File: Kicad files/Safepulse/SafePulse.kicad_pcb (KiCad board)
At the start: 4 copper layers, 40.6 x 20.8 mm, 90 parts, among them J1 Conn_01x03_Male, Q1 FQT7N10L, Q2 BC846A, Q3 MMBT3906, Q4 MMBT3906, U1 TS4061AILT-1.25, U2 74HC14, U3 TLV27L1DBVT, U33 MAX9910EXK+T, U4 CD14538BM

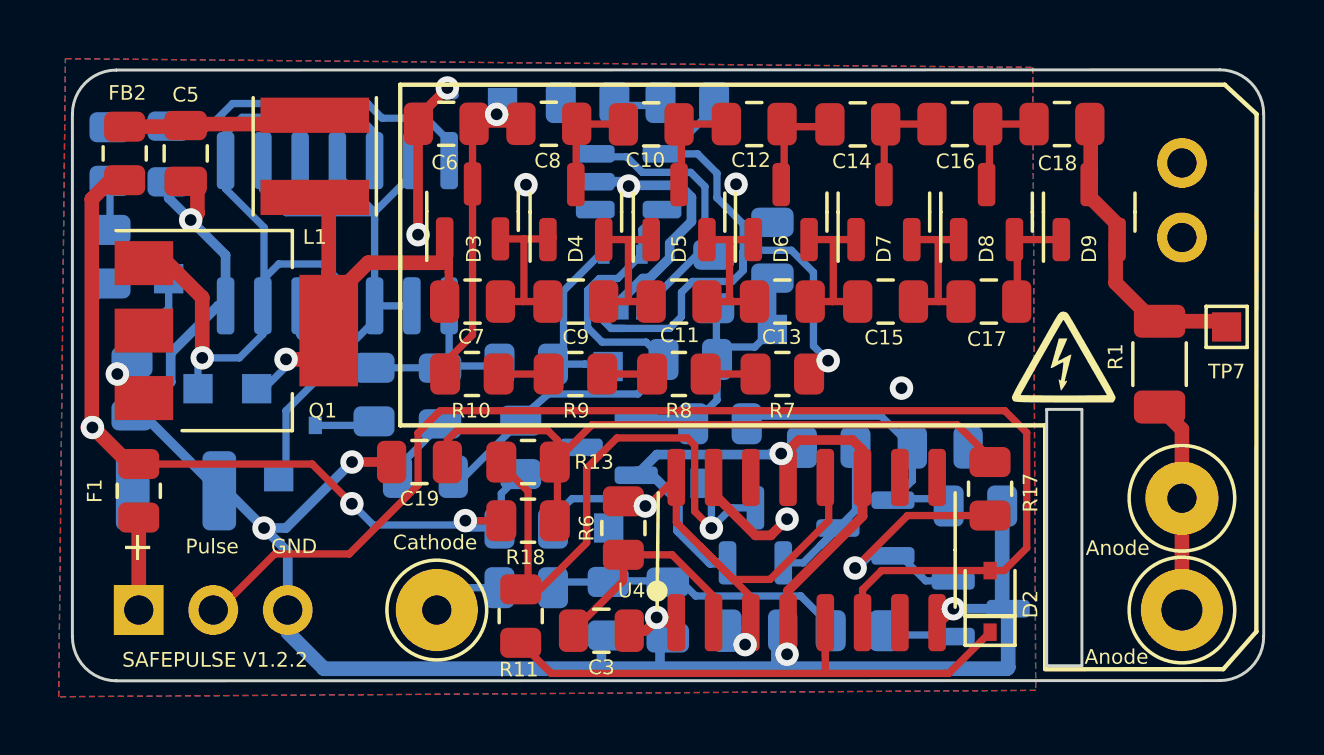
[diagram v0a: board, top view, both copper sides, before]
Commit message: Updated with Gerbers
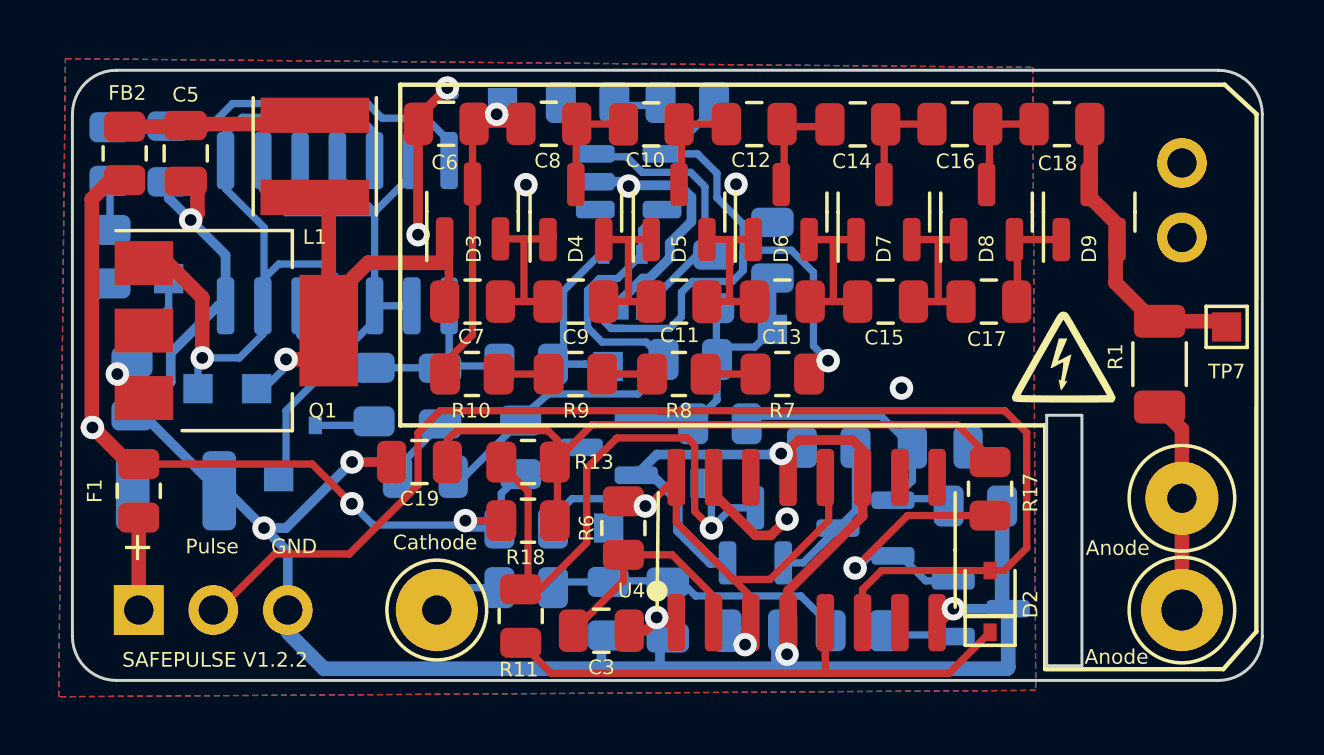
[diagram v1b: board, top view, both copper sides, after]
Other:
- outline, holes or cut-outs redrawn
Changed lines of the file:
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@@
   (gr_line (start 165.52 57.658) (end 137.414 57.658) (layer "F.SilkS") (width 0.15))
   (gr_line (start 165.52 57.658) (end 166.604 58.658) (layer "F.SilkS") (width 0.15))
-  (gr_arc (start 165.347 76.47) (end 166.847 76.47) (angle 90) (layer "Edge.Cuts") (width 0.1))
-  (gr_line (start 165.347 77.97) (end 127.738 77.978) (layer "Edge.Cuts") (width 0.1))
-  (gr_line (start 166.847 58.65) (end 166.847 76.47) (layer "Edge.Cuts") (width 0.1))
-  (gr_arc (start 165.347 58.65) (end 165.347 57.15) (angle 90) (layer "Edge.Cuts") (width 0.1))
-  (gr_rect (start 159.45 68.725) (end 160.65 77.465) (layer "Edge.Cuts") (width 0.1) (fill none))
-  (gr_arc (start 127.738 76.478) (end 127.738 77.978) (angle 90) (layer "Edge.Cuts") (width 0.1))
-  (gr_line (start 127.738 57.158) (end 165.347 57.15) (layer "Edge.Cuts") (width 0.1))
-  (gr_line (start 126.238 76.478) (end 126.238 58.658) (layer "Edge.Cuts") (width 0.1))
-  (gr_arc (start 127.738 58.658) (end 126.238 58.658) (angle 90) (layer "Edge.Cuts") (width 0.1))
+  (gr_arc (start 165.3 76.465) (end 166.8 76.465) (angle 90) (layer "Edge.Cuts") (width 0.1))
+  (gr_line (start 165.3 77.965) (end 127.738 77.965) (layer "Edge.Cuts") (width 0.1))
+  (gr_line (start 166.8 58.665) (end 166.8 76.465) (layer "Edge.Cuts") (width 0.1))
+  (gr_arc (start 127.738 58.665) (end 126.238 58.665) (angle 90) (layer "Edge.Cuts") (width 0.1))
+  (gr_arc (start 165.3 58.665) (end 165.3 57.165) (angle 90) (layer "Edge.Cuts") (width 0.1))
+  (gr_rect (start 159.45 68.925) (end 160.65 77.465) (layer "Edge.Cuts") (width 0.1) (fill none))
+  (gr_line (start 165.3 57.165) (end 127.738 57.165) (layer "Edge.Cuts") (width 0.1))
+  (gr_arc (start 127.738 76.465) (end 126.238 76.465) (angle -90) (layer "Edge.Cuts") (width 0.1))
+  (gr_line (start 126.238 76.465) (end 126.238 58.665) (layer "Edge.Cuts") (width 0.1))
   (gr_text "GND\n" (at 133.925 73.7) (layer "B.SilkS")
     (effects (font (size 0.5 0.5) (thickness 0.1)) (justify mirror))
